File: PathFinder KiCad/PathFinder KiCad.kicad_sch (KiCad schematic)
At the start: 11 parts, among them J1 Conn_01x02_Socket, SW1 SW_Push, SW2 SW_Push, SW3 SW_Push, U1 XIAO-RP2040-DIP

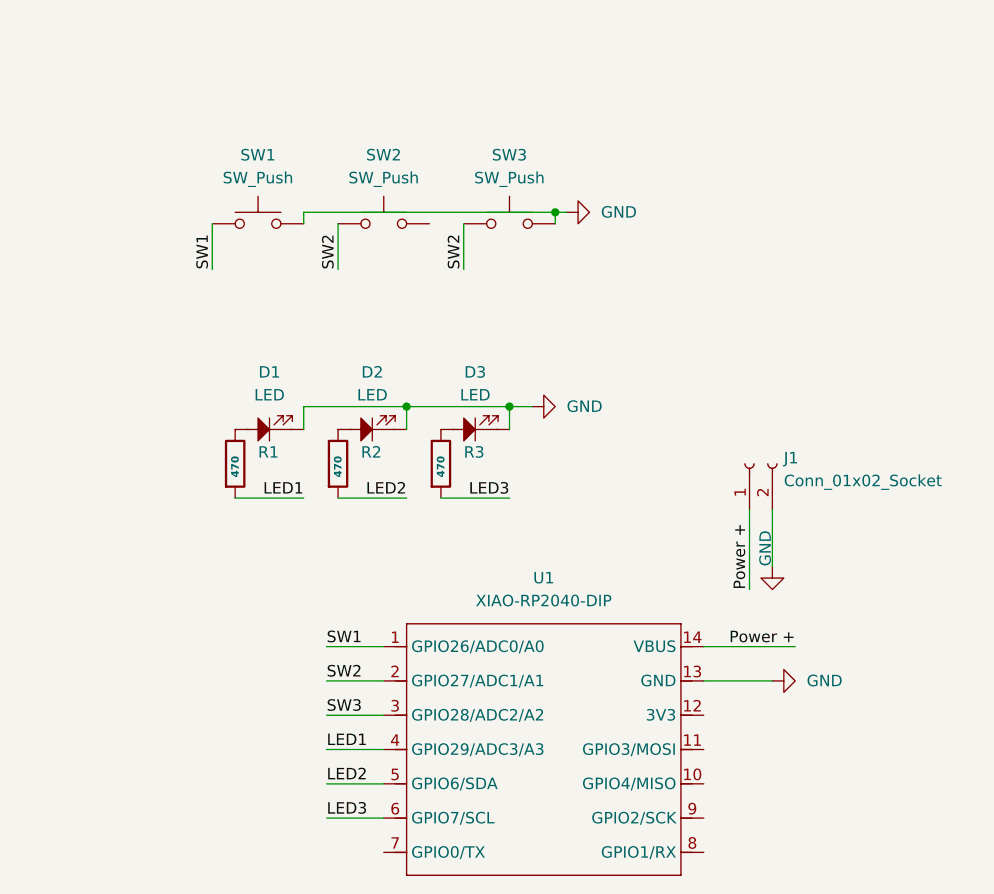
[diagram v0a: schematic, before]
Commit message: KiCad Fix
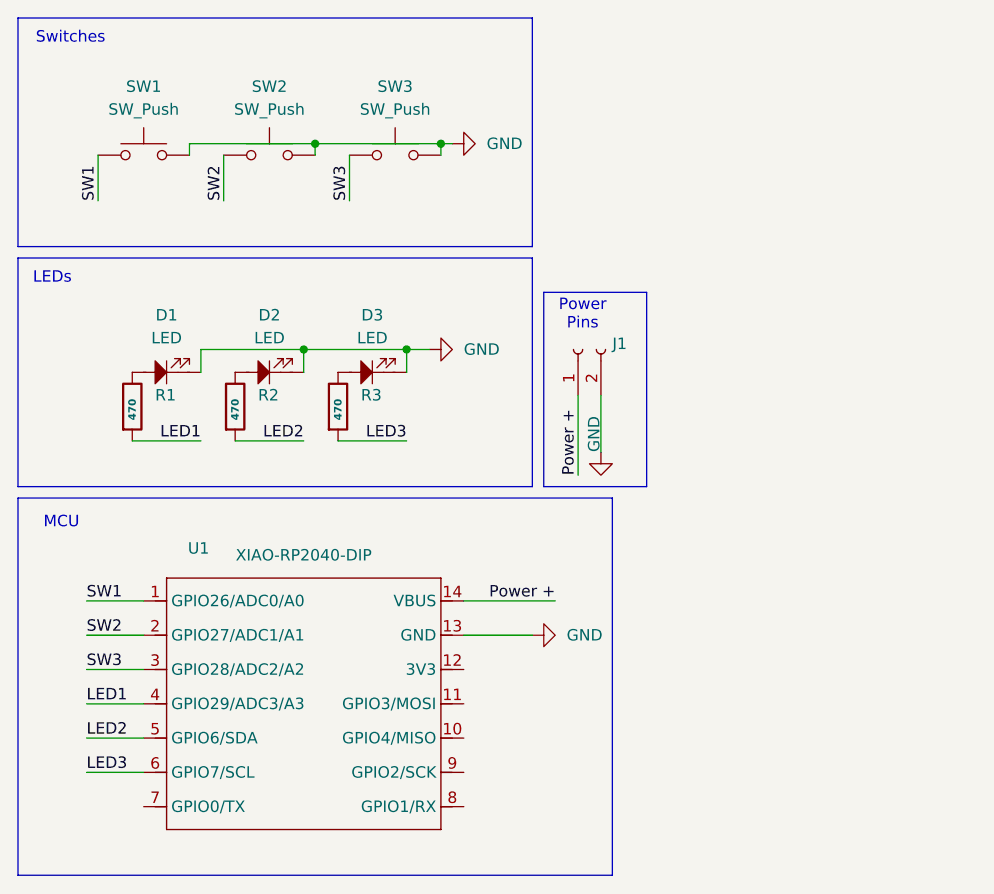
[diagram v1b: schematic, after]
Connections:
- net GND: now also SW2.2
- net SW2: no longer SW3.1
- net SW3: now also SW3.1
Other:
- note added: "LEDs"
- note added: "MCU"
- note added: "Power Pins"
- note added: "Switches"
- moved on the sheet: D1, D2, D3, J1, R1, R2, R3, SW1, SW2, SW3, U1
